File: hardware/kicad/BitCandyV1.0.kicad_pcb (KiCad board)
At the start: 2 copper layers, 59.6 x 27.9 mm, 19 parts

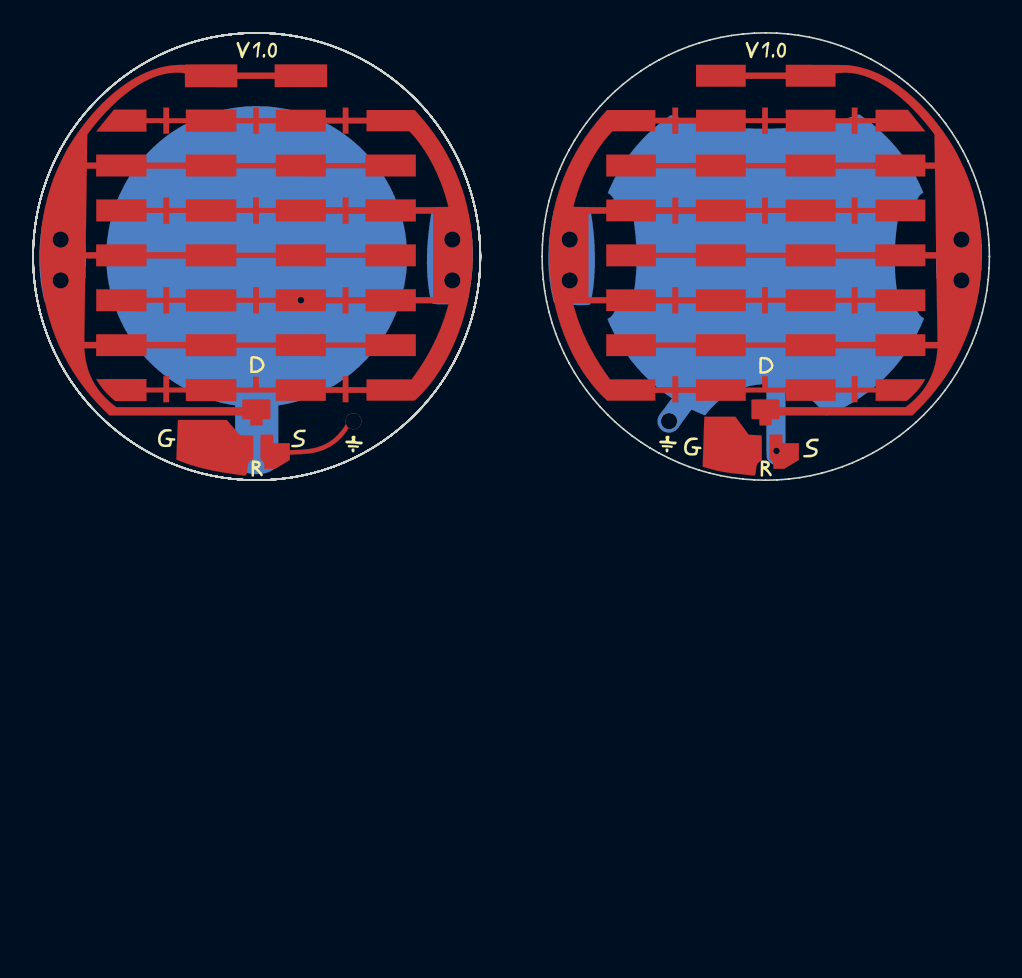
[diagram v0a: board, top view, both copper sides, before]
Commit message: bitCandy , plotted
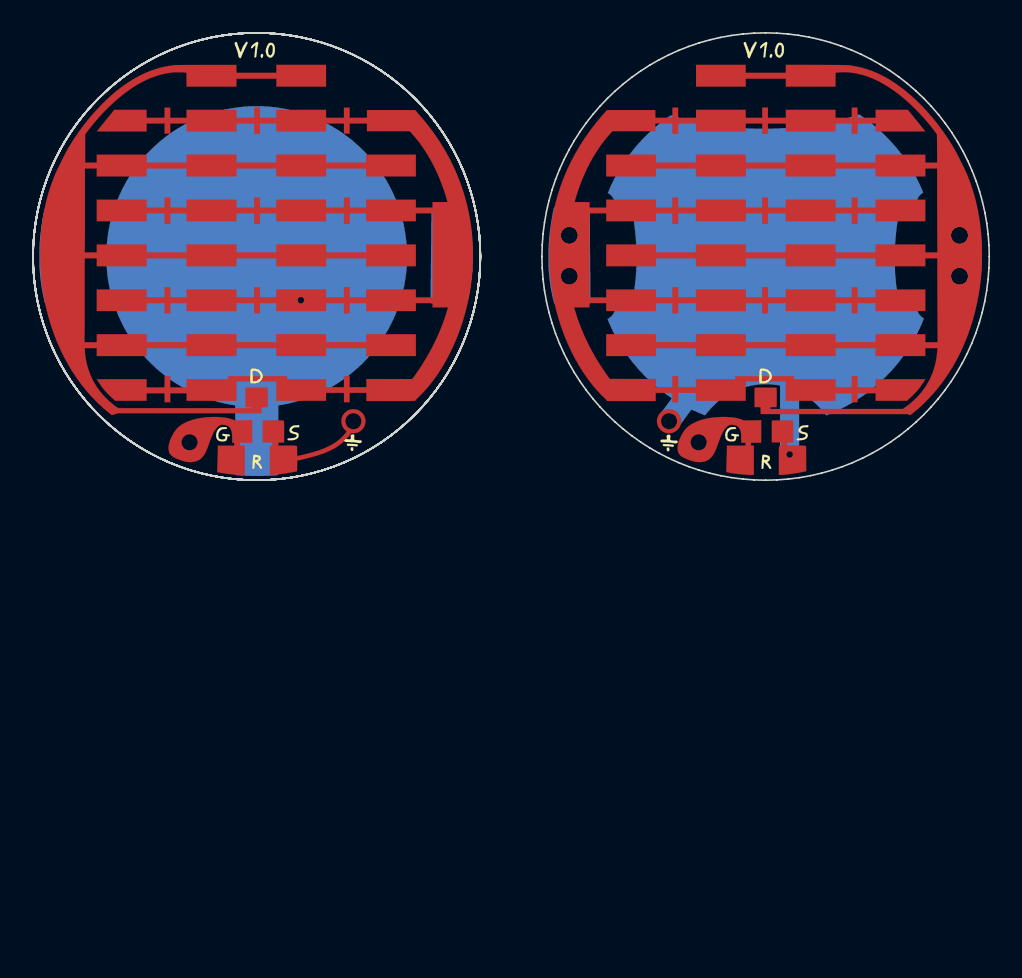
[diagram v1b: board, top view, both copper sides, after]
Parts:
- removed the ? at (13.9, 32.5)
- removed the ? at (19.7, -11.6)
- removed the ? at (-4.73, -11.6)
- removed the ? at (-12.0, -11.6)
- removed the ? at (-36.5, -11.6)
- removed the ? at (8.17, 1.59)
- removed the ? at (19.7, -9.05)
- removed the ? at (-4.73, -9.05)
- removed the ? at (-12.0, -9.05)
- removed the ? at (-36.5, -9.05)
- removed the ? at (-21.5, -7.81)
- removed the ? at (1.47, -0.27)
- removed the ? at (-18.2, -0.27)
- removed the G*** at (0.00, 0.00) (x6)
- added ?: , Wire_Pads:SolderWirePad_single_0-8mmDrill, F.Cu at (8.99, 1.81)
- added ? (x2): , Wire_Pads:SolderWirePad_single_0-8mmDrill, F.Cu at (-4.76, -9.31)
- added ? (x2): , Wire_Pads:SolderWirePad_single_0-8mmDrill, F.Cu at (19.6, -11.9)
- added ? (x2): , Wire_Pads:SolderWirePad_single_0-8mmDrill, F.Cu at (-4.76, -11.9)
- added ?: , Wire_Pads:SolderWirePad_single_0-8mmDrill, F.Cu at (3.31, 1.05)
- added ?: , Wire_Pads:SolderWirePad_single_0-8mmDrill, F.Cu at (-28.4, 1.05)
- added ? (x2): , Wire_Pads:SolderWirePad_single_0-8mmDrill, F.Cu at (19.6, -9.31)
- added ?: , Wire_Pads:SolderWirePad_single_0-8mmDrill, F.Cu at (-21.5, -7.81)
- added ?: , Wire_Pads:SolderWirePad_single_0-8mmDrill, F.Cu at (1.47, -0.27)
- added ?: , Wire_Pads:SolderWirePad_single_0-8mmDrill, F.Cu at (-18.2, -0.27)
- added G*** (x6): LOGO, LOGO, F.Cu at (0.00, 0.00)
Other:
- outline, holes or cut-outs redrawn
